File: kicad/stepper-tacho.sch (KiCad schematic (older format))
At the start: 3 parts

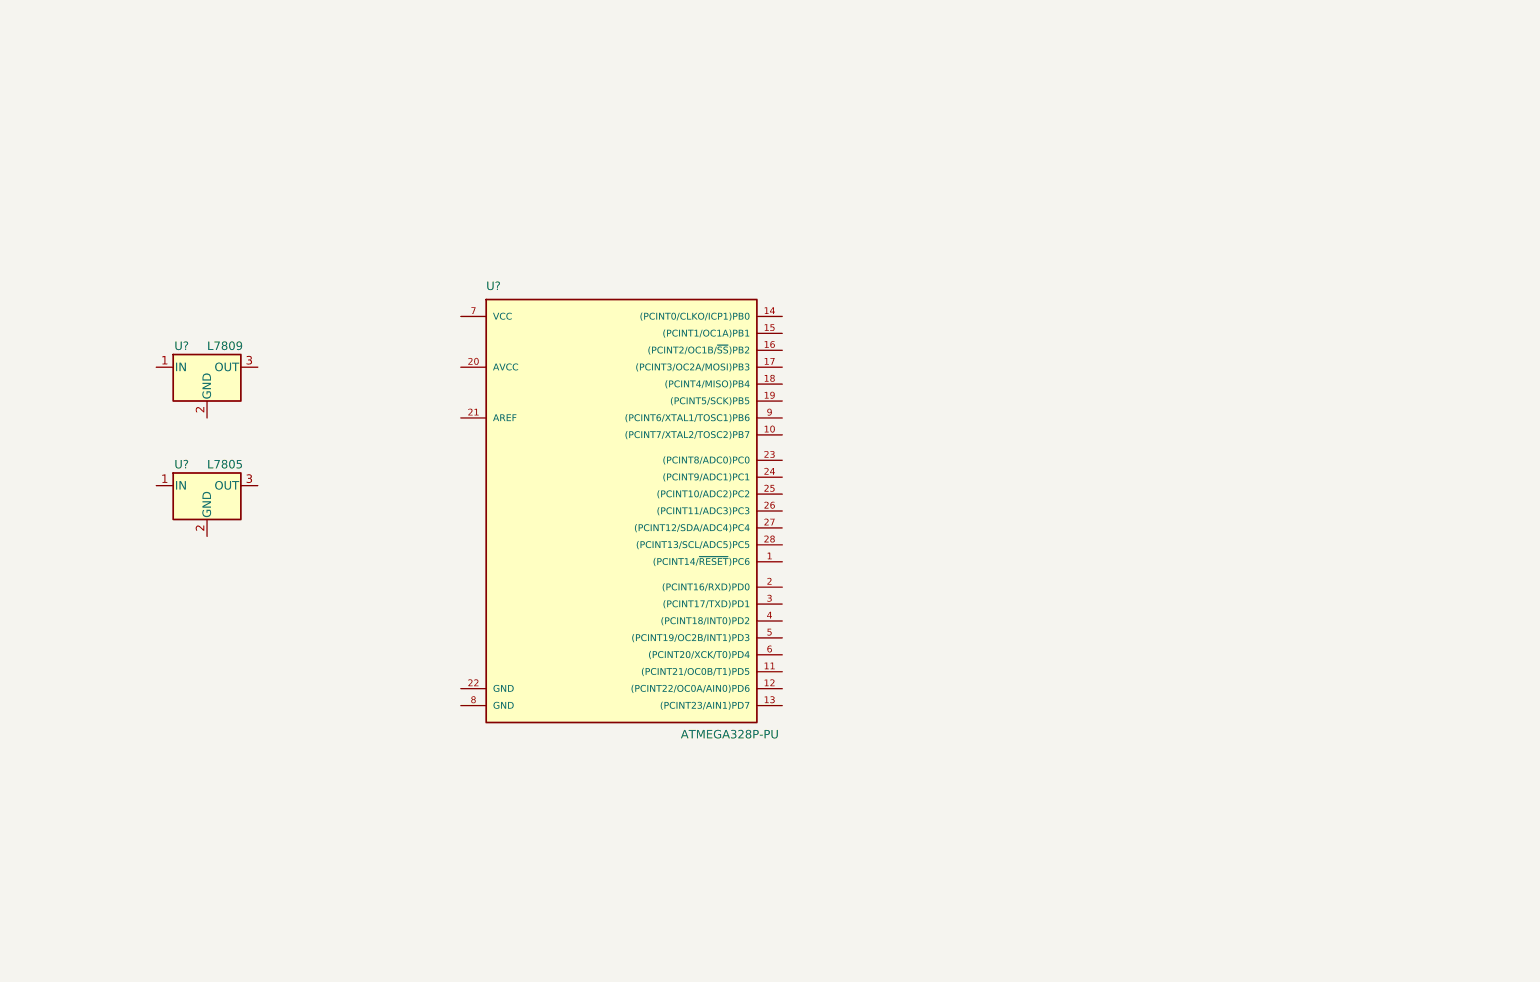
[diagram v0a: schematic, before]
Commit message: pcb配置
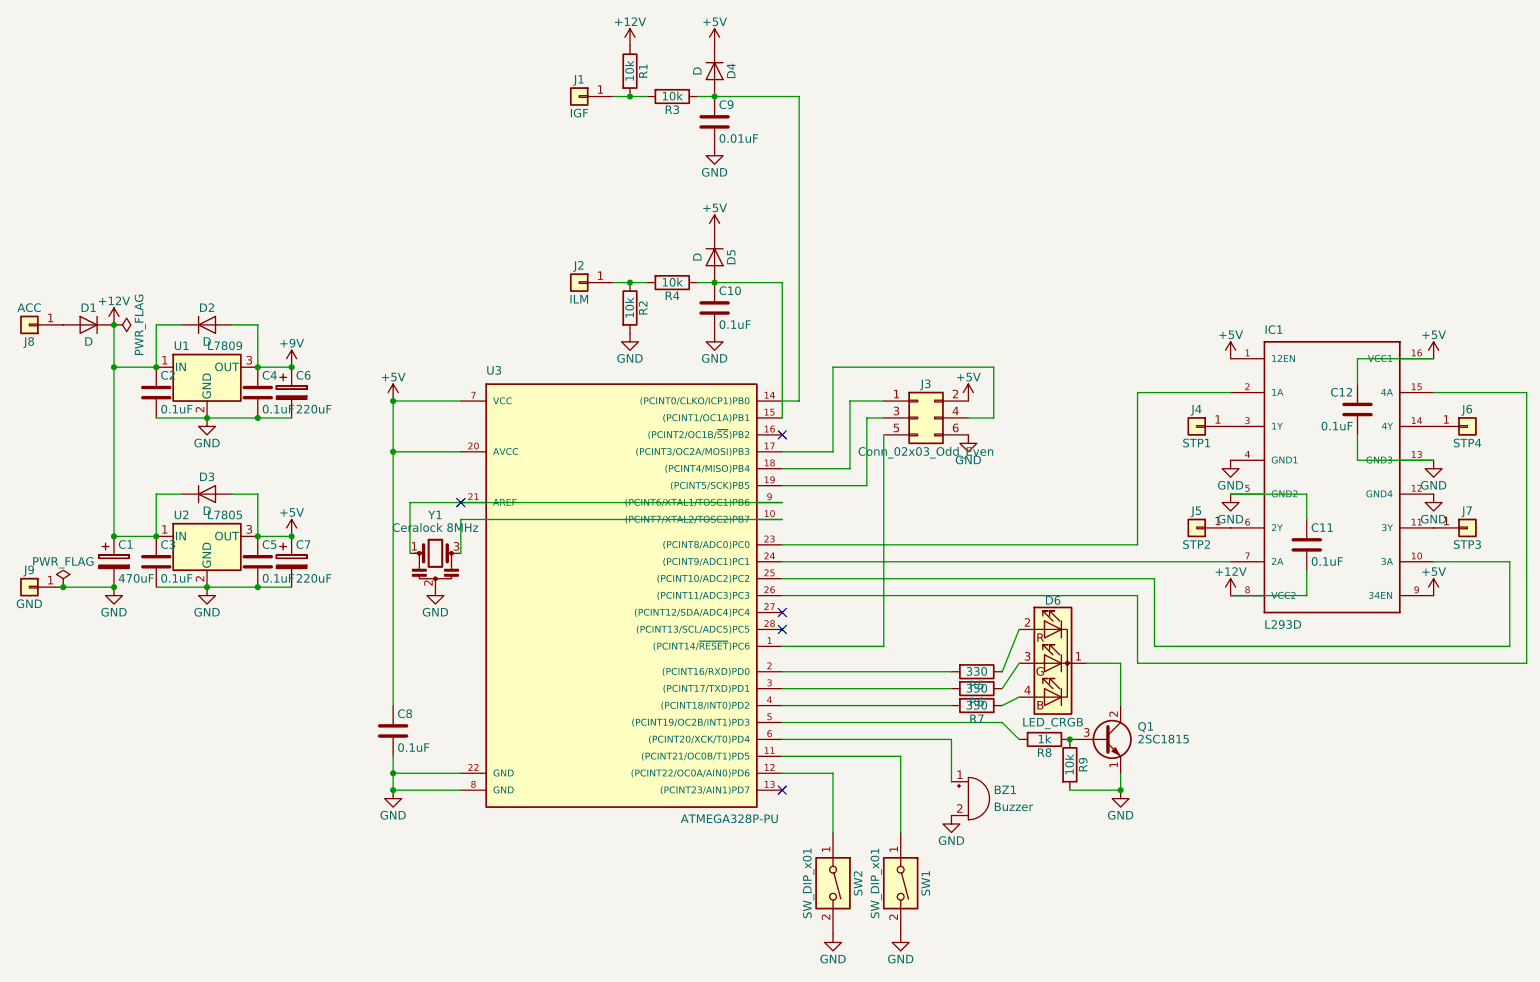
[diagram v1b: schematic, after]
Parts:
- added BZ1: Buzzer, Pin_Headers:Pin_Header_Straight_1x02_Pitch2.54mm, symbol Buzzer
- added C1: 470uF, Capacitors_THT:CP_Radial_D10.0mm_P5.00mm, symbol CP
- added C10, C11, C12, C2, C3, C4, C5, C8: 0.1uF, Capacitors_THT:C_Disc_D5.0mm_W2.5mm_P2.50mm, symbol C
- added C6, C7: 220uF, Capacitors_THT:CP_Radial_D8.0mm_P3.50mm, symbol CP
- added C9: 0.01uF, Capacitors_THT:C_Disc_D5.0mm_W2.5mm_P2.50mm, symbol C
- added D1: D, Diodes_THT:D_A-405_P5.08mm_Vertical_KathodeUp, symbol D
- added D2, D3, D4, D5: D, Diodes_THT:D_T-1_P10.16mm_Horizontal, symbol D
- added D6: LED_CRGB, Pin_Headers:Pin_Header_Straight_1x04_Pitch2.54mm, symbol LED_CRGB
- added IC1: L293D, Housings_DIP:DIP-16_W7.62mm, symbol L293D
- added J1: IGF, Pin_Headers:Pin_Header_Straight_1x01_Pitch2.54mm, symbol Conn_01x01
- added J2: ILM, Pin_Headers:Pin_Header_Straight_1x01_Pitch2.54mm, symbol Conn_01x01
- added J3: Conn_02x03_Odd_Even, Pin_Headers:Pin_Header_Straight_2x03_Pitch2.54mm, symbol Conn_02x03_Odd_Even
- added J4: STP1, Pin_Headers:Pin_Header_Straight_1x01_Pitch2.54mm, symbol Conn_01x01
- added J5: STP2, Pin_Headers:Pin_Header_Straight_1x01_Pitch2.54mm, symbol Conn_01x01
- added J6: STP4, Pin_Headers:Pin_Header_Straight_1x01_Pitch2.54mm, symbol Conn_01x01
- added J7: STP3, Pin_Headers:Pin_Header_Straight_1x01_Pitch2.54mm, symbol Conn_01x01
- added J8: ACC, Pin_Headers:Pin_Header_Straight_1x01_Pitch2.54mm, symbol Conn_01x01
- added J9: GND, Pin_Headers:Pin_Header_Straight_1x01_Pitch2.54mm, symbol Conn_01x01
- added Q1: 2SC1815, TO_SOT_Packages_THT:TO-92_Molded_Narrow, symbol 2SC1815
- added R1, R2, R3, R4, R9: 10k, Resistors_THT:R_Axial_DIN0207_L6.3mm_D2.5mm_P7.62mm_Horizontal, symbol R
- added R5, R6, R7: 330, Resistors_THT:R_Axial_DIN0207_L6.3mm_D2.5mm_P7.62mm_Horizontal, symbol R
- added R8: 1k, Resistors_THT:R_Axial_DIN0207_L6.3mm_D2.5mm_P7.62mm_Horizontal, symbol R
- added SW1, SW2: SW_DIP_x01, Pin_Headers:Pin_Header_Straight_1x02_Pitch2.54mm, symbol SW_DIP_x01
- added Y1: Ceralock 8MHz, Crystals:Resonator_muRata_CSTLSxxxG-3pin_w8.0mm_h3.0mm, symbol Resonator
- U1, U2: renamed from U?; footprint (none) -> TO_SOT_Packages_THT:TO-220-3_Vertical
- U3: renamed from U?; footprint DIL28 -> Housings_DIP:DIP-28_W7.62mm
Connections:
- net at U3.1 ((PCINT14/~RESET~)PC6): now also J3.5 (Pin_5)
- net at U3.10 ((PCINT7/XTAL2/TOSC2)PB7): now also Y1.3
- net at U3.11 ((PCINT21/OC0B/T1)PD5): now also SW1.1
- net at U3.12 ((PCINT22/OC0A/AIN0)PD6): now also SW2.1
- net at U3.14 ((PCINT0/CLKO/ICP1)PB0): now also C9.1, D4.2 (A), R3.1
- net at U3.15 ((PCINT1/OC1A)PB1): now also C10.1, D5.2 (A), R4.1
- net at U3.17 ((PCINT3/OC2A/MOSI)PB3): now also J3.4 (Pin_4)
- net at U3.18 ((PCINT4/MISO)PB4): now also J3.1 (Pin_1)
- net at U3.19 ((PCINT5/SCK)PB5): now also J3.3 (Pin_3)
- net at U3.2 ((PCINT16/RXD)PD0): now also R5.2
- net +5V: now reaches U3.20 (AVCC)
- net +5V: now also U2.3 (OUT), U3.7 (VCC), C12.1, C5.1, C7.1, C8.1, D3.2 (A), D4.1 (K), D5.1 (K), IC1.1 (12EN), IC1.16 (VCC1), IC1.9 (34EN), J3.2 (Pin_2)
- net GND: now reaches U3.22 (GND)
- net GND: now also U1.2 (GND), U2.2 (GND), U3.8 (GND), BZ1.2 (+), C1.2, C10.2, C11.1, C12.2, C2.2, C3.2, C4.2, C5.2, C6.2, C7.2, C8.2, C9.2, IC1.12 (GND4), IC1.13 (GND3), IC1.4 (GND1), IC1.5 (GND2), J3.6 (Pin_6), J9.1 (Pin_1), Q1.1 (E), R2.2, R9.2, SW1.2, SW2.2, Y1.2
- net at U3.23 ((PCINT8/ADC0)PC0): now also IC1.2 (1A)
- net at U3.24 ((PCINT9/ADC1)PC1): now also IC1.7 (2A)
- net at U3.25 ((PCINT10/ADC2)PC2): now also IC1.10 (3A)
- net at U3.26 ((PCINT11/ADC3)PC3): now also IC1.15 (4A)
- net at U3.3 ((PCINT17/TXD)PD1): now also R6.2
- net at U3.4 ((PCINT18/INT0)PD2): now also R7.2
- net at U3.5 ((PCINT19/OC2B/INT1)PD3): now also R8.2
- net at U3.6 ((PCINT20/XCK/T0)PD4): now also BZ1.1 (-)
- net at U3.9 ((PCINT6/XTAL1/TOSC1)PB6): now also Y1.1
- net +12V: now reaches U1.1 (IN)
- net +12V: now also U2.1 (IN), C1.1, C11.2, C2.1, C3.1, D1.1 (K), D2.1 (K), D3.1 (K), IC1.8 (VCC2), R1.1
- net +9V: now reaches U1.3 (OUT)
- net +9V: now also C4.1, C6.1, D2.2 (A)
- new net: J2.1 (Pin_1), R2.1, R4.2
- new net: J1.1 (Pin_1), R1.2, R3.2
- new net: IC1.11 (3Y), J7.1 (Pin_1)
- new net: IC1.14 (4Y), J6.1 (Pin_1)
- new net: IC1.3 (1Y), J4.1 (Pin_1)
- new net: IC1.6 (2Y), J5.1 (Pin_1)
- new net: D1.2 (A), J8.1 (Pin_1)
- new net: D6.2 (RA), R5.1
- new net: D6.3 (GA), R6.1
- new net: D6.4 (BA), R7.1
- new net: D6.1 (K), Q1.2 (C)
- new net: Q1.3 (B), R8.1, R9.1
- no-connect marks 0 -> 5
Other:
- moved on the sheet: U2, U3
